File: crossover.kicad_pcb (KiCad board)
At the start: 2 copper layers, 78 parts, among them J1 Power In, J2 Line In, J3 Tweeter Out, J4 Sub Out, U1 TL072, U2 TL072, U3 TL072, U4 TL072, U5 TL072, U6 TL072, U7 TL072

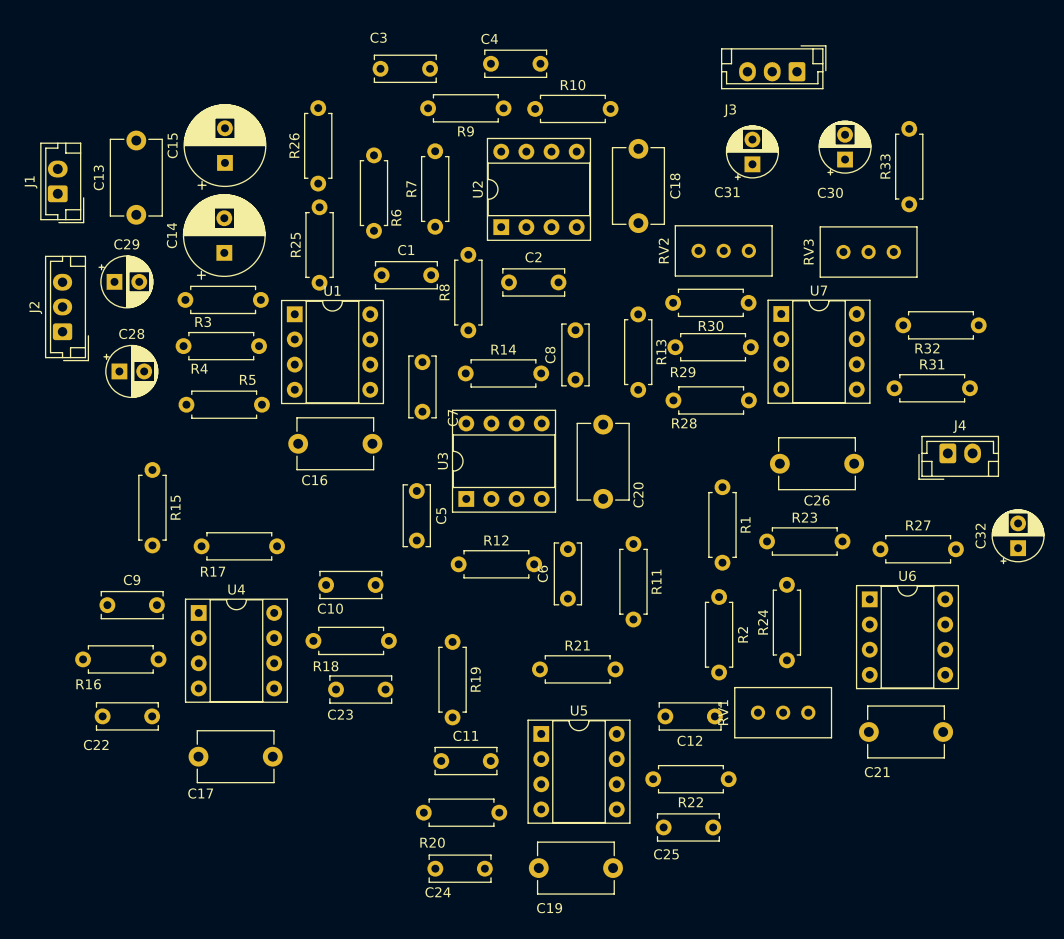
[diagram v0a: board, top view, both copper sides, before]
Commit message: Set boundaries, labels
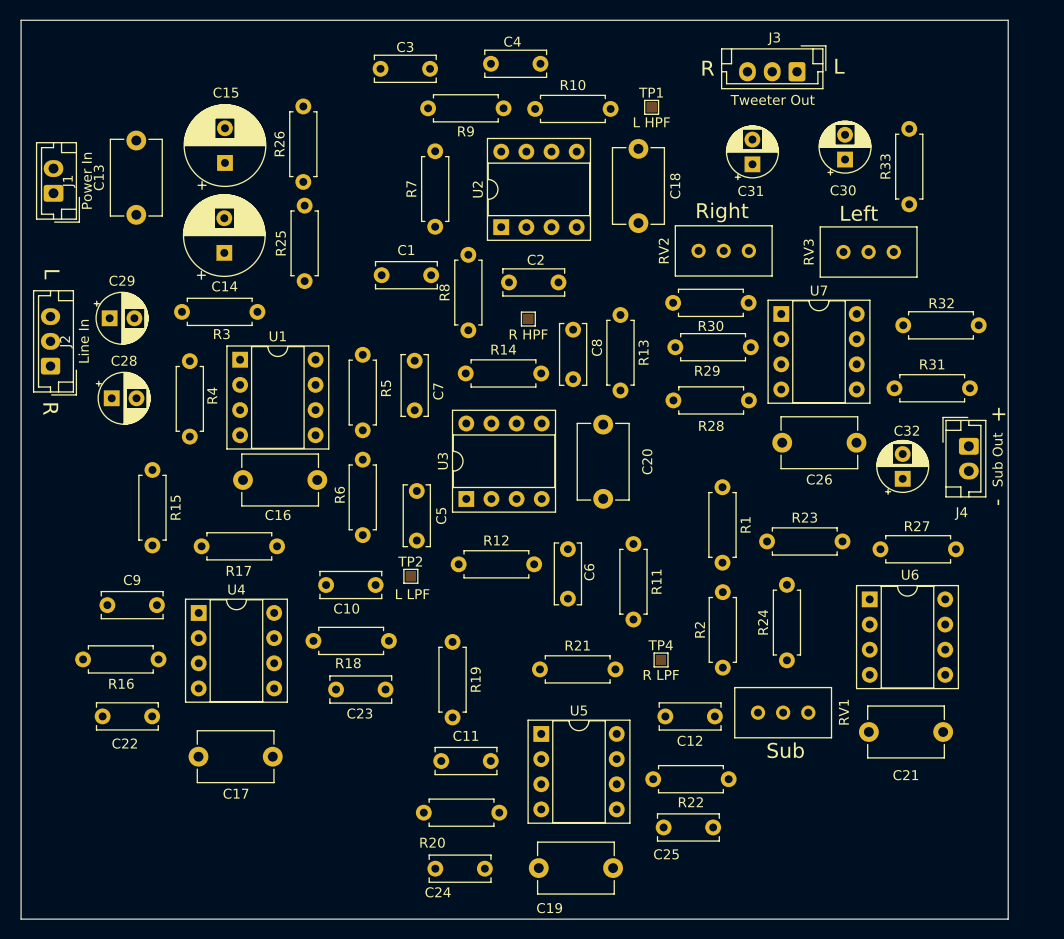
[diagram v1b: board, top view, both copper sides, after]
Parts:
- added TP1: L HPF, TestPoint:TestPoint_Pad_1.0x1.0mm, F.Cu at (126.5, 35.3)
- added TP2: L LPF, TestPoint:TestPoint_Pad_1.0x1.0mm, F.Cu at (102.2, 82.6)
- added TP3: R HPF, TestPoint:TestPoint_Pad_1.0x1.0mm, F.Cu at (114.0, 56.6)
- added TP4: R LPF, TestPoint:TestPoint_Pad_1.0x1.0mm, F.Cu at (127.4, 91.1)
- moved R6 23.1 mm to (97.3, 70.8), turned to -90 degrees
- moved C32 13.6 mm to (151.8, 72.8)
- moved R5 10.5 mm to (97.3, 67.9), turned to 90 degrees
- moved U1 7.18 mm to (84.9, 60.8)
- moved R4 7.15 mm to (79.9, 60.9), turned to -90 degrees
- moved C16 6.66 mm to (92.7, 72.9)
- moved C29 3.71 mm to (71.8, 56.6)
- moved J2 3.68 mm to (65.8, 61.4)
- moved C28 2.82 mm to (72.0, 64.6)
- moved J4 2.24 mm to (158.5, 69.5), turned to -90 degrees
- moved C26 2.13 mm to (147.2, 69.1)
- moved R13 1.79 mm to (123.3, 56.2)
- moved R25 1.51 mm to (91.4, 52.8)
- moved R26 1.51 mm to (91.3, 42.8)
- moved R3 1.26 mm to (86.7, 55.9)
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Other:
- board outline added: 99.7 x 90.8 mm
- board text added: "+"
- board text added: "-"
- board text added: "L"
- board text added: "Left"
- board text added: "R"
- board text added: "Right"
- board text added: "Sub"
